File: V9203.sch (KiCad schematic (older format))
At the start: 54 parts, among them J1 RJ45, J4 Screw_Terminal_1x04, J6 CONN_01X06, J7 GS3, J8 GS3, U1 V9203, Y1 Crystal_GND24

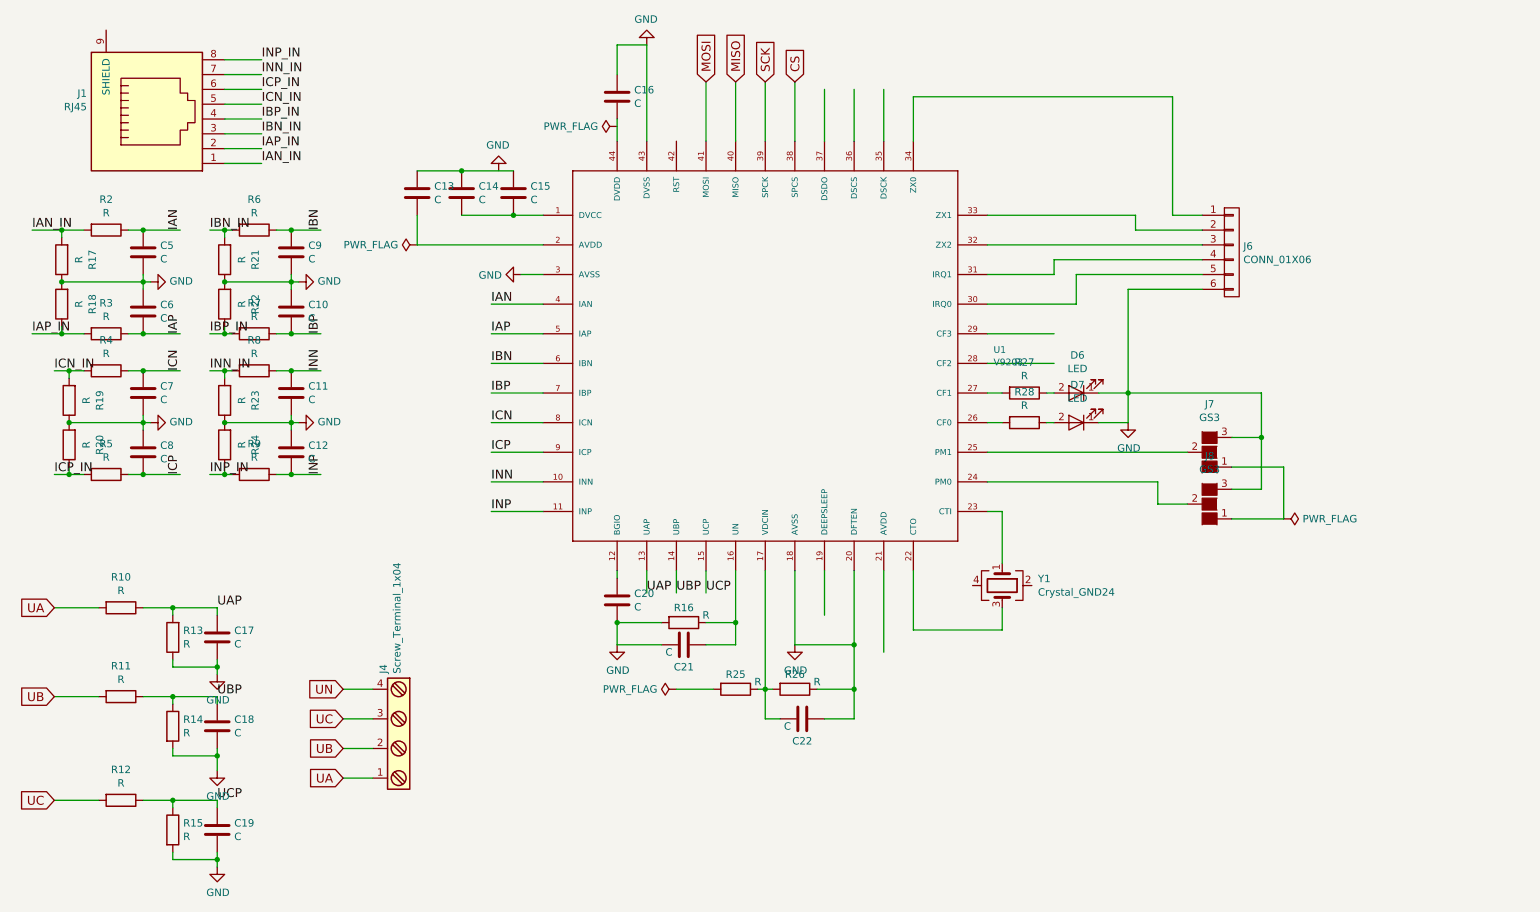
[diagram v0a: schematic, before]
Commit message: Neaten up parts layout
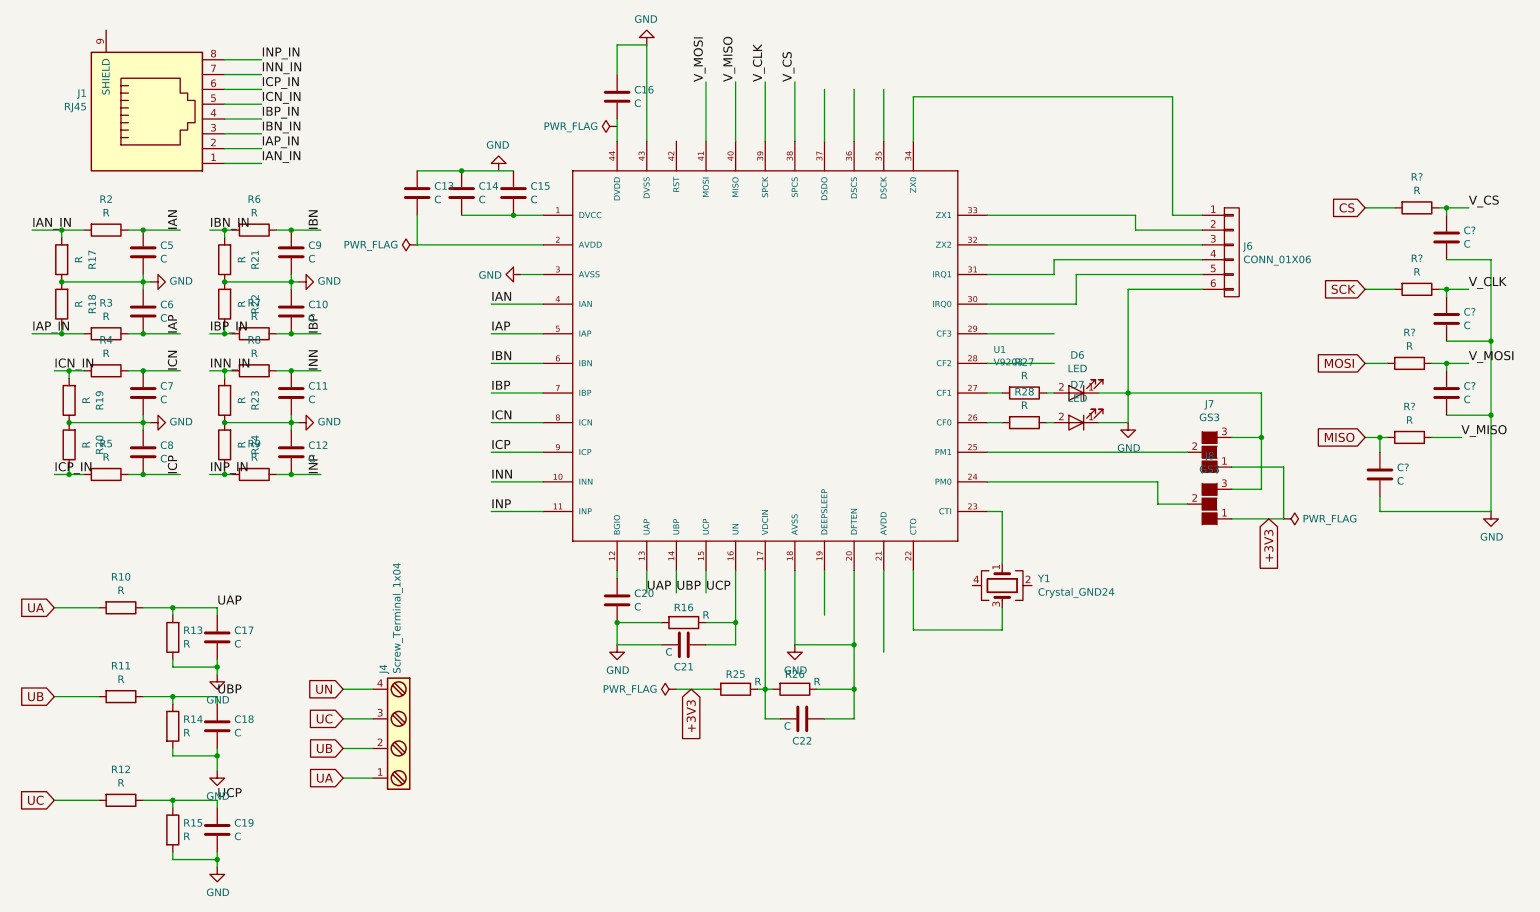
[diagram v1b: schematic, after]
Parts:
- added C? (x4): C, Capacitors_SMD:C_0402, symbol C
- added R? (x4): R, Resistors_SMD:R_0402, symbol R
- R17, R18, R19, R20, R21, R22, R23, R24: footprint Resistors_SMD:R_0402 -> Resistors_SMD:R_0603
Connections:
- net labels added: +3V3, V_CLK, V_CS, V_MISO, V_MOSI
- wire segments 149 -> 167
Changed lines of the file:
@@
 Text Label 3850 4500 0    60   ~ 0
 INP
-Text GLabel 5300 1600 1    60   Input ~ 0
-MOSI
-Text GLabel 5500 1600 1    60   Input ~ 0
-MISO
-Text GLabel 5700 1600 1    60   Input ~ 0
-SCK
-Text GLabel 5900 1600 1    60   Input ~ 0
-CS
 $Comp
 L LED D7
@@
 F 0 "R17" V 743 2800 50  0000 C CNN
 F 1 "R" V 834 2800 50  0000 C CNN
-F 2 "Resistors_SMD:R_0402" V -1670 650 50  0001 C CNN
+F 2 "Resistors_SMD:R_0603" V -1670 650 50  0001 C CNN
 F 3 "" H -1600 650 50  0001 C CNN
 	1    950  2800
@@
 F 0 "R18" V 743 3100 50  0000 C CNN
 F 1 "R" V 834 3100 50  0000 C CNN
-F 2 "Resistors_SMD:R_0402" V -1670 950 50  0001 C CNN
+F 2 "Resistors_SMD:R_0603" V -1670 950 50  0001 C CNN
 F 3 "" H -1600 950 50  0001 C CNN
 	1    950  3100
@@
 F 0 "R21" V 1843 2800 50  0000 C CNN
 F 1 "R" V 1934 2800 50  0000 C CNN
-F 2 "Resistors_SMD:R_0402" V -570 650 50  0001 C CNN
+F 2 "Resistors_SMD:R_0603" V -570 650 50  0001 C CNN
 F 3 "" H -500 650 50  0001 C CNN
 	1    2050 2800
@@
 F 0 "R22" V 1843 3100 50  0000 C CNN
 F 1 "R" V 1934 3100 50  0000 C CNN
-F 2 "Resistors_SMD:R_0402" V -570 950 50  0001 C CNN
+F 2 "Resistors_SMD:R_0603" V -570 950 50  0001 C CNN
 F 3 "" H -500 950 50  0001 C CNN
 	1    2050 3100
@@
 F 0 "R19" V 793 3750 50  0000 C CNN
 F 1 "R" V 884 3750 50  0000 C CNN
-F 2 "Resistors_SMD:R_0402" V -1620 1600 50  0001 C CNN
+F 2 "Resistors_SMD:R_0603" V -1620 1600 50  0001 C CNN
 F 3 "" H -1550 1600 50  0001 C CNN
 	1    1000 3750
@@
 F 0 "R20" V 793 4050 50  0000 C CNN
 F 1 "R" V 884 4050 50  0000 C CNN
-F 2 "Resistors_SMD:R_0402" V -1620 1900 50  0001 C CNN
+F 2 "Resistors_SMD:R_0603" V -1620 1900 50  0001 C CNN
 F 3 "" H -1550 1900 50  0001 C CNN
 	1    1000 4050
@@
 F 0 "R23" V 1843 3750 50  0000 C CNN
 F 1 "R" V 1934 3750 50  0000 C CNN
-F 2 "Resistors_SMD:R_0402" V -570 1600 50  0001 C CNN
+F 2 "Resistors_SMD:R_0603" V -570 1600 50  0001 C CNN
 F 3 "" H -500 1600 50  0001 C CNN
 	1    2050 3750
@@
 F 0 "R24" V 1843 4050 50  0000 C CNN
 F 1 "R" V 1934 4050 50  0000 C CNN
-F 2 "Resistors_SMD:R_0402" V -570 1900 50  0001 C CNN
+F 2 "Resistors_SMD:R_0603" V -570 1900 50  0001 C CNN
 F 3 "" H -500 1900 50  0001 C CNN
 	1    2050 4050
@@
 	0    1    1    0
 $EndComp
+Text GLabel 5200 5700 3    60   Input ~ 0
++3V3
+Text GLabel 9100 4550 3    60   Input ~ 0
++3V3
+$Comp
+L R R?
+U 1 1 58FE5B05
+P 10100 2450
+F 0 "R?" V 9893 2450 50  0000 C CNN
+F 1 "R" V 9984 2450 50  0000 C CNN
+F 2 "Resistors_SMD:R_0402" V 7480 300 50  0001 C CNN
+F 3 "" H 7550 300 50  0001 C CNN
+	1    10100 2450
+	0    1    1    0
+$EndComp
+$Comp
+L C C?
+U 1 1 58FE5BE7
+P 10300 2650
+F 0 "C?" H 10415 2696 50  0000 L CNN
+F 1 "C" H 10415 2605 50  0000 L CNN
+F 2 "Capacitors_SMD:C_0402" H 8738 -450 50  0001 C CNN
+F 3 "" H 8700 -300 50  0001 C CNN
+	1    10300 2650
+	1    0    0    -1
+$EndComp
+$Comp
+L R R?
+U 1 1 58FE5CF5
+P 10100 3000
+F 0 "R?" V 9893 3000 50  0000 C CNN
+F 1 "R" V 9984 3000 50  0000 C CNN
+F 2 "Resistors_SMD:R_0402" V 7480 850 50  0001 C CNN
+F 3 "" H 7550 850 50  0001 C CNN
+	1    10100 3000
+	0    1    1    0
+$EndComp
+$Comp
+L C C?
+U 1 1 58FE5D9B
+P 10300 3200
+F 0 "C?" H 10415 3246 50  0000 L CNN
+F 1 "C" H 10415 3155 50  0000 L CNN
+F 2 "Capacitors_SMD:C_0402" H 8738 100 50  0001 C CNN
+F 3 "" H 8700 250 50  0001 C CNN
+	1    10300 3200
+	1    0    0    -1
+$EndComp
+$Comp
+L R R?
+U 1 1 58FE5E43
+P 10050 3500
+F 0 "R?" V 9843 3500 50  0000 C CNN
+F 1 "R" V 9934 3500 50  0000 C CNN
+F 2 "Resistors_SMD:R_0402" V 7430 1350 50  0001 C CNN
+F 3 "" H 7500 1350 50  0001 C CNN
+	1    10050 3500
+	0    1    1    0
+$EndComp
+$Comp
+L C C?
+U 1 1 58FE5EEF
+P 10300 3700
+F 0 "C?" H 10415 3746 50  0000 L CNN
+F 1 "C" H 10415 3655 50  0000 L CNN
+F 2 "Capacitors_SMD:C_0402" H 8738 600 50  0001 C CNN
+F 3 "" H 8700 750 50  0001 C CNN
+	1    10300 3700
+	1    0    0    -1
+$EndComp
+$Comp
+L C C?
+U 1 1 58FE5F95
+P 9850 4250
+F 0 "C?" H 9965 4296 50  0000 L CNN
+F 1 "C" H 9965 4205 50  0000 L CNN
+F 2 "Capacitors_SMD:C_0402" H 8288 1150 50  0001 C CNN
+F 3 "" H 8250 1300 50  0001 C CNN
+	1    9850 4250
+	1    0    0    -1
+$EndComp
+$Comp
+L R R?
+U 1 1 58FE6045
+P 10050 4000
+F 0 "R?" V 9843 4000 50  0000 C CNN
+F 1 "R" V 9934 4000 50  0000 C CNN
+F 2 "Resistors_SMD:R_0402" V 7430 1850 50  0001 C CNN
+F 3 "" H 7500 1850 50  0001 C CNN
+	1    10050 4000
+	0    1    1    0
+$EndComp
+Text Label 5300 1600 1    60   ~ 0
+V_MOSI
+Text Label 5500 1600 1    60   ~ 0
+V_MISO
+Text Label 5700 1600 1    60   ~ 0
+V_CLK
+Text Label 5900 1600 1    60   ~ 0
+V_CS
+Wire Wire Line
+	10250 2450 10450 2450
+Wire Wire Line
+	10300 2450 10300 2500
+Connection ~ 10300 2450
+Wire Wire Line
+	10250 3000 10450 3000
+Wire Wire Line
+	10300 3000 10300 3050
+Connection ~ 10300 3000
+Wire Wire Line
+	10200 3500 10450 3500
+Wire Wire Line
+	10300 3500 10300 3550
+Connection ~ 10300 3500
+Wire Wire Line
+	9850 4100 9850 4000
+Connection ~ 9850 4000
+Wire Wire Line
+	10200 4000 10400 4000
+$Comp
+L GND #PWR?
+U 1 1 58FE85DB
+P 10600 4500
+F 0 "#PWR?" H 5800 2250 50  0001 C CNN
+F 1 "GND" H 10605 4327 50  0000 C CNN
+F 2 "" H 5800 2500 50  0001 C CNN
+F 3 "" H 5800 2500 50  0001 C CNN
+	1    10600 4500
+	1    0    0    -1
+$EndComp
+Wire Wire Line
+	9850 4400 9850 4500
+Wire Wire Line
+	9850 4500 10600 4500
+Wire Wire Line
+	10300 3850 10600 3850
+Wire Wire Line
+	10600 4500 10600 2800
+Wire Wire Line
+	10600 3350 10300 3350
+Connection ~ 10600 3850
+Wire Wire Line
+	10600 2800 10300 2800
+Connection ~ 10600 3350
+Wire Wire Line
+	9950 2450 9750 2450
+Wire Wire Line
+	9950 3000 9750 3000
+Wire Wire Line
+	9900 3500 9750 3500
+Wire Wire Line
+	9900 4000 9750 4000
+Text Label 10450 2450 0    60   ~ 0
+V_CS
+Text Label 10450 3000 0    60   ~ 0
+V_CLK
+Text Label 10450 3500 0    60   ~ 0
+V_MOSI
+Text Label 10400 4000 0    60   ~ 0
+V_MISO
+Text GLabel 9750 2450 0    60   Input ~ 0
+CS
+Text GLabel 9750 3000 0    60   Input ~ 0
+SCK
+Text GLabel 9750 3500 0    60   Input ~ 0
+MOSI
+Text GLabel 9750 4000 0    60   Input ~ 0
+MISO
 $EndSCHEMATC
